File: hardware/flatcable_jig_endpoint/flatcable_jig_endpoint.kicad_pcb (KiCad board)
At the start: 2 copper layers, 2 parts

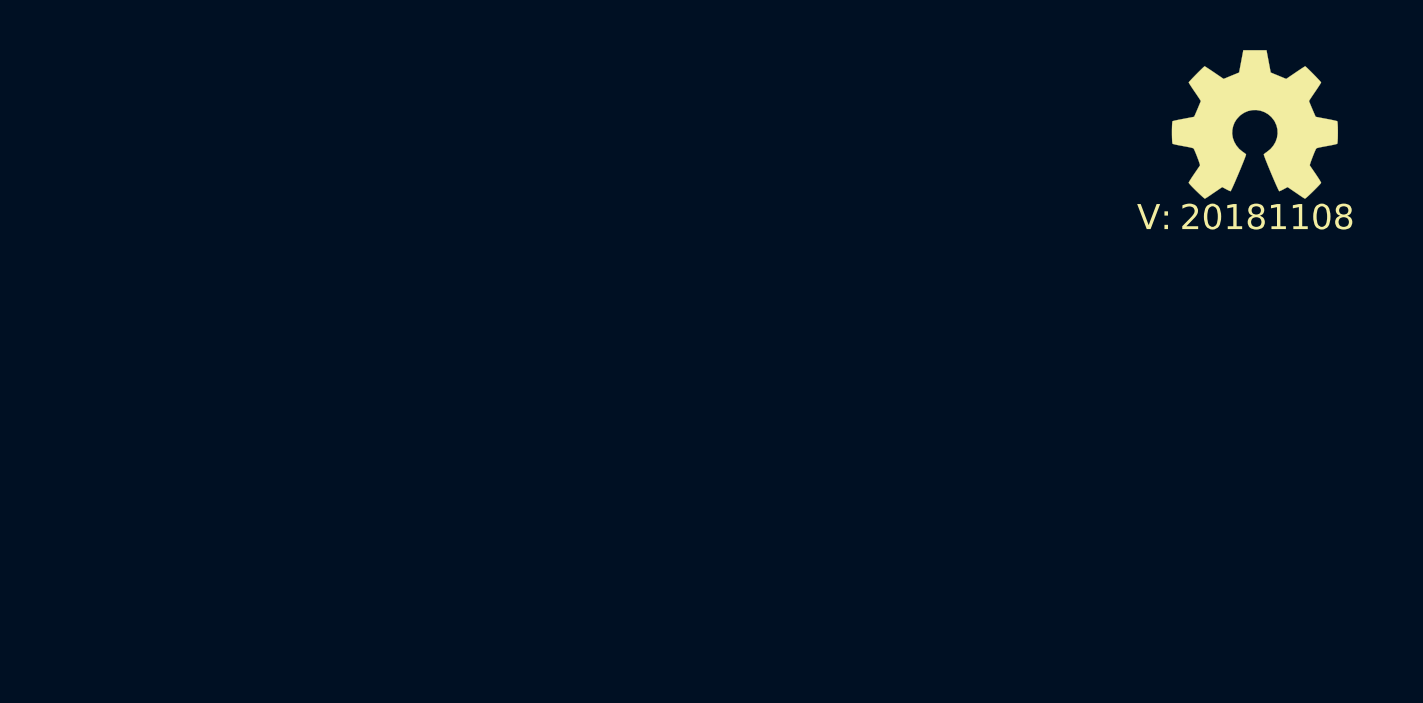
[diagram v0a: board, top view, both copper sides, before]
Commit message: started layout, still need to add the endpad connections
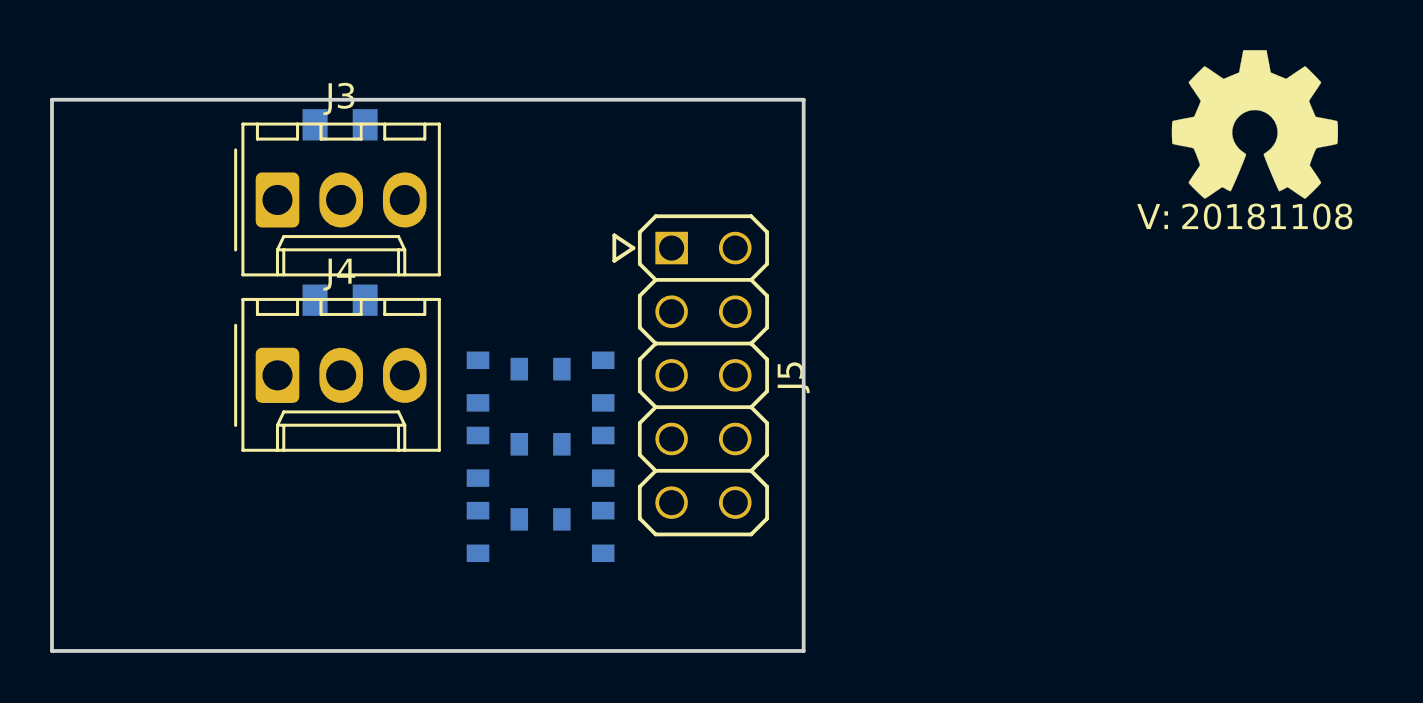
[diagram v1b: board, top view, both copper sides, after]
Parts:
- added C1: C, SquantorRcl:C_0805, B.Cu at (111.5, 101.0)
- added C2: C, SquantorRcl:C_0805, B.Cu at (111.5, 108.0)
- added J3: Conn_01x03, Connector_Molex:Molex_KK-254_AE-6410-03A_1x03_P2.54mm_Vertical, F.Cu at (109.0, 104.0)
- added J4: Conn_01x03, Connector_Molex:Molex_KK-254_AE-6410-03A_1x03_P2.54mm_Vertical, F.Cu at (109.0, 111.0)
- added J5: Conn_02x05_Odd_Even, SquantorConnectors:Header-0254-2X05-H010, F.Cu at (126.0, 111.0)
- added R1: R, SquantorRcl:R_0603_hand, B.Cu at (117.0, 111.2)
- added R2: R, SquantorRcl:R_0603_hand, B.Cu at (117.0, 114.2)
- added R3: R, SquantorRcl:R_0603_hand, B.Cu at (117.0, 117.2)
- added R4: R, SquantorRcl:R_0603_hand, B.Cu at (119.5, 110.8)
- added R5: R, SquantorRcl:R_0603_hand, B.Cu at (119.5, 113.8)
- added R6: R, SquantorRcl:R_0603_hand, B.Cu at (119.5, 116.8)
- added R7: R, SquantorRcl:R_0603_hand, B.Cu at (122.0, 111.2)
- added R8: R, SquantorRcl:R_0603_hand, B.Cu at (122.0, 114.2)
- added R9: R, SquantorRcl:R_0603_hand, B.Cu at (122.0, 117.2)
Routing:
- added copper zone on F.Cu, net GND
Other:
- board outline added: 30 x 22 mm
